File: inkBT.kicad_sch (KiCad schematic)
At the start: 34 parts, among them J1 AudioJack2_Ground, J2 Conn_01x10, J3 Conn_01x06, U1 LM2596S-5, U2 ESP32-WROOM-32, U3 PCM5102A, U5 LM2596S-3.3, U6 ME6211C33M5, U7 ME6211C33M5

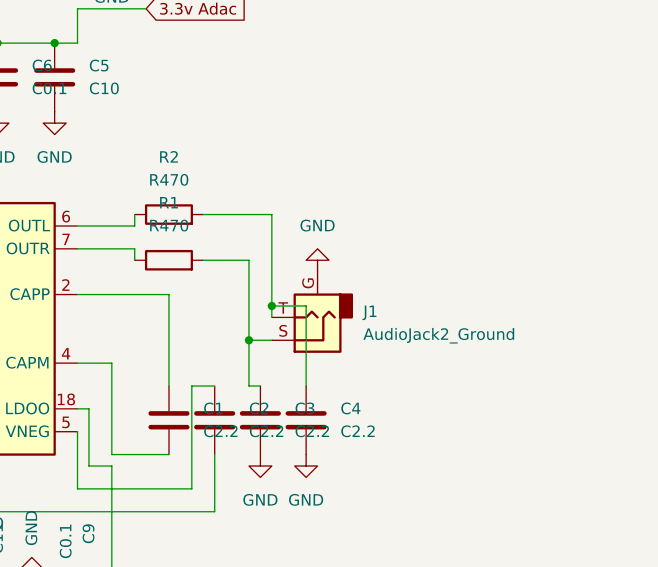
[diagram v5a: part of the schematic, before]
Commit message: a
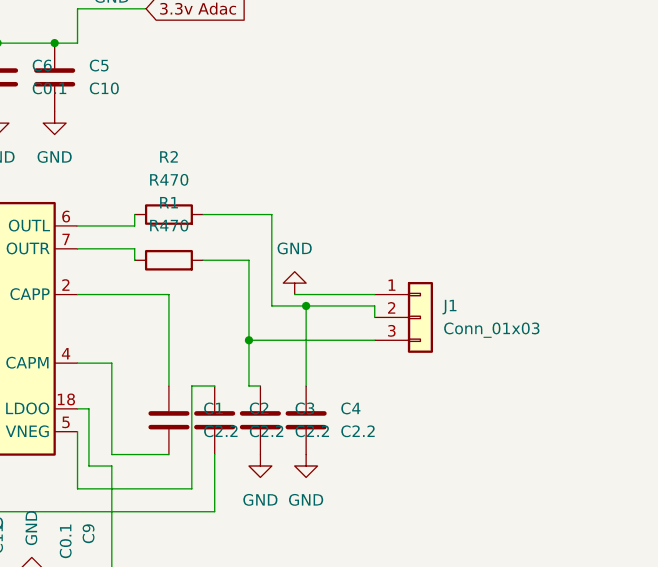
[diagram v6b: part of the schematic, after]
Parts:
- removed J1: AudioJack2_Ground, Connector_PinSocket_1.00mm:PinSocket_1x03_P1.00mm_Vertical, symbol Connector_Audio:AudioJack2_Ground
- added J1: Conn_01x03, Connector_PinHeader_2.00mm:PinHeader_1x03_P2.00mm_Vertical, symbol Connector_Generic:Conn_01x03
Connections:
- net GND: now also J1.1 (Pin_1)
- net at C3.1, R1.2: now also J1.3 (Pin_3)
- net at C4.1, R2.2: now also J1.2 (Pin_2)
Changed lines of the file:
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@@
 	)
 	(junction
+		(at 157.48 104.14)
+		(diameter 0)
+		(color 0 0 0 0)
+	)
+	(junction
 		(at 123.19 74.93)
 		(diameter 0)
@@
 	)
 	(junction
-		(at 153.67 104.14)
-		(diameter 0)
-		(color 0 0 0 0)
-	)
-	(junction
 		(at 129.54 74.93)
 		(diameter 0)
@@
 	(wire
 		(pts
+			(xy 165.1 104.14) (xy 157.48 104.14)
+		)
+		(stroke
+			(width 0)
+			(type default)
+		)
+	)
+	(wire
+		(pts
 			(xy 121.92 81.28) (xy 119.38 81.28)
 		)
@@
 	(wire
 		(pts
+			(xy 156.21 102.87) (xy 165.1 102.87)
+		)
+		(stroke
+			(width 0)
+			(type default)
+		)
+	)
+	(wire
+		(pts
 			(xy 127 40.64) (xy 127 22.86)
 		)
@@
 	(wire
 		(pts
-			(xy 153.67 104.14) (xy 153.67 105.41)
+			(xy 165.1 104.14) (xy 165.1 105.41)
 		)
 		(stroke
@@
 	(wire
 		(pts
+			(xy 157.48 104.14) (xy 153.67 104.14)
+		)
+		(stroke
+			(width 0)
+			(type default)
+		)
+	)
+	(wire
+		(pts
 			(xy 116.84 123.19) (xy 116.84 127)
 		)
@@
 	(wire
 		(pts
-			(xy 151.13 107.95) (xy 153.67 107.95)
+			(xy 151.13 107.95) (xy 165.1 107.95)
 		)
 		(stroke
@@
 	(wire
 		(pts
-			(xy 157.48 104.14) (xy 153.67 104.14)
-		)
-		(stroke
-			(width 0)
-			(type default)
-		)
-	)
-	(wire
-		(pts
 			(xy 97.79 100.33) (xy 106.68 100.33)
 		)
@@
 		(lib_name "GND_1")
 		(lib_id "power:GND")
-		(at 158.75 100.33 180)
+		(at 156.21 102.87 180)
 		(unit 1)
 		(body_style 1)
@@
 		(fields_autoplaced yes)
 		(property "Reference" "#PWR05"
-			(at 158.75 93.98 0)
+			(at 156.21 96.52 0)
 			(hide yes)
 			(show_name no)
@@
 		)
 		(property "Value" "GND"
-			(at 158.75 95.25 0)
+			(at 156.21 97.79 0)
 			(show_name no)
 			(do_not_autoplace no)
@@
 		)
 		(property "Footprint" ""
-			(at 158.75 100.33 0)
+			(at 156.21 102.87 0)
 			(hide yes)
 			(show_name no)
@@
 		)
 		(property "Datasheet" ""
-			(at 158.75 100.33 0)
+			(at 156.21 102.87 0)
 			(hide yes)
 			(show_name no)
@@
 		)
 		(property "Description" "Power symbol creates a global label with name \"GND\" , ground"
-			(at 158.75 100.33 0)
+			(at 156.21 102.87 0)
 			(hide yes)
 			(show_name no)
@@
 	)
 	(symbol
+		(lib_id "Connector_Generic:Conn_01x03")
+		(at 170.18 105.41 0)
+		(unit 1)
+		(body_style 1)
+		(exclude_from_sim no)
+		(in_bom yes)
+		(on_board yes)
+		(in_pos_files yes)
+		(dnp no)
+		(fields_autoplaced yes)
+		(property "Reference" "J1"
+			(at 172.72 104.1399 0)
+			(show_name no)
+			(do_not_autoplace no)
+			(effects
+				(font
+					(size 1.27 1.27)
+				)
+				(justify left)
+			)
+		)
+		(property "Value" "Conn_01x03"
+			(at 172.72 106.6799 0)
+			(show_name no)
+			(do_not_autoplace no)
+			(effects
+				(font
+					(size 1.27 1.27)
+				)
+				(justify left)
+			)
+		)
+		(property "Footprint" "Connector_PinHeader_2.00mm:PinHeader_1x03_P2.00mm_Vertical"
+			(at 170.18 105.41 0)
+			(hide yes)
+			(show_name no)
+			(do_not_autoplace no)
+			(effects
+				(font
+					(size 1.27 1.27)
+				)
+			)
+		)
+		(property "Datasheet" ""
+			(at 170.18 105.41 0)
+			(hide yes)
+			(show_name no)
+			(do_not_autoplace no)
+			(effects
+				(font
+					(size 1.27 1.27)
+				)
+			)
+		)
+		(property "Description" "Generic connector, single row, 01x03, script generated (kicad-library-utils/schlib/autogen/connector/)"
+			(at 170.18 105.41 0)
+			(hide yes)
+			(show_name no)
+			(do_not_autoplace no)
+			(effects
+				(font
+					(size 1.27 1.27)
+				)
+			)
+		)
+		(pin "2"
+		)
+		(pin "1"
+		)
+		(pin "3"
+		)
+		(instances
+			(project "inkBT"
+				(path "/d639bd58-f563-44ff-a906-a8a044dd820d"
+					(reference "J1")
+					(unit 1)
+				)
+			)
+		)
+	)
+	(symbol
 		(lib_id "Device:R")
 		(at 142.24 93.98 90)
@@
 					(unit 1)
 				)
-			)
-		)
-	)
-	(symbol
-		(lib_id "Connector_Audio:AudioJack2_Ground")
-		(at 158.75 105.41 180)
-		(unit 1)
-		(body_style 1)
-		(exclude_from_sim no)
-		(in_bom yes)
-		(on_board yes)
-		(in_pos_files yes)
-		(dnp no)
-		(fields_autoplaced yes)
-		(property "Reference" "J1"
-			(at 163.83 104.775 0)
-			(show_name no)
-			(do_not_autoplace no)
-			(effects
-				(font
-					(size 1.27 1.27)
-				)
-				(justify right)
-			)
-		)
-		(property "Value" "AudioJack2_Ground"
-			(at 163.83 107.315 0)
-			(show_name no)
-			(do_not_autoplace no)
-			(effects
-				(font
-					(size 1.27 1.27)
-				)
-				(justify right)
-			)
-		)
-		(property "Footprint" "Connector_PinSocket_1.00mm:PinSocket_1x03_P1.00mm_Vertical"
-			(at 158.75 105.41 0)
-			(hide yes)
-			(show_name no)
-			(do_not_autoplace no)
-			(effects
-				(font
-					(size 1.27 1.27)
-				)
-			)
-		)
-		(property "Datasheet" ""
-			(at 158.75 105.41 0)
-			(hide yes)
-			(show_name no)
-			(do_not_autoplace no)
-			(effects
-				(font
-					(size 1.27 1.27)
-				)
-			)
-		)
-		(property "Description" ""
-			(at 158.75 105.41 0)
-			(show_name no)
-			(do_not_autoplace no)
-			(effects
-				(font
-					(size 1.27 1.27)
-				)
-			)
-		)
-		(pin "S"
-		)
-		(pin "G"
-		)
-		(pin "T"
-		)
-		(instances
-			(project "inkBT"
-				(path "/d639bd58-f563-44ff-a906-a8a044dd820d"
-					(reference "J1")
-					(unit 1)
-				)

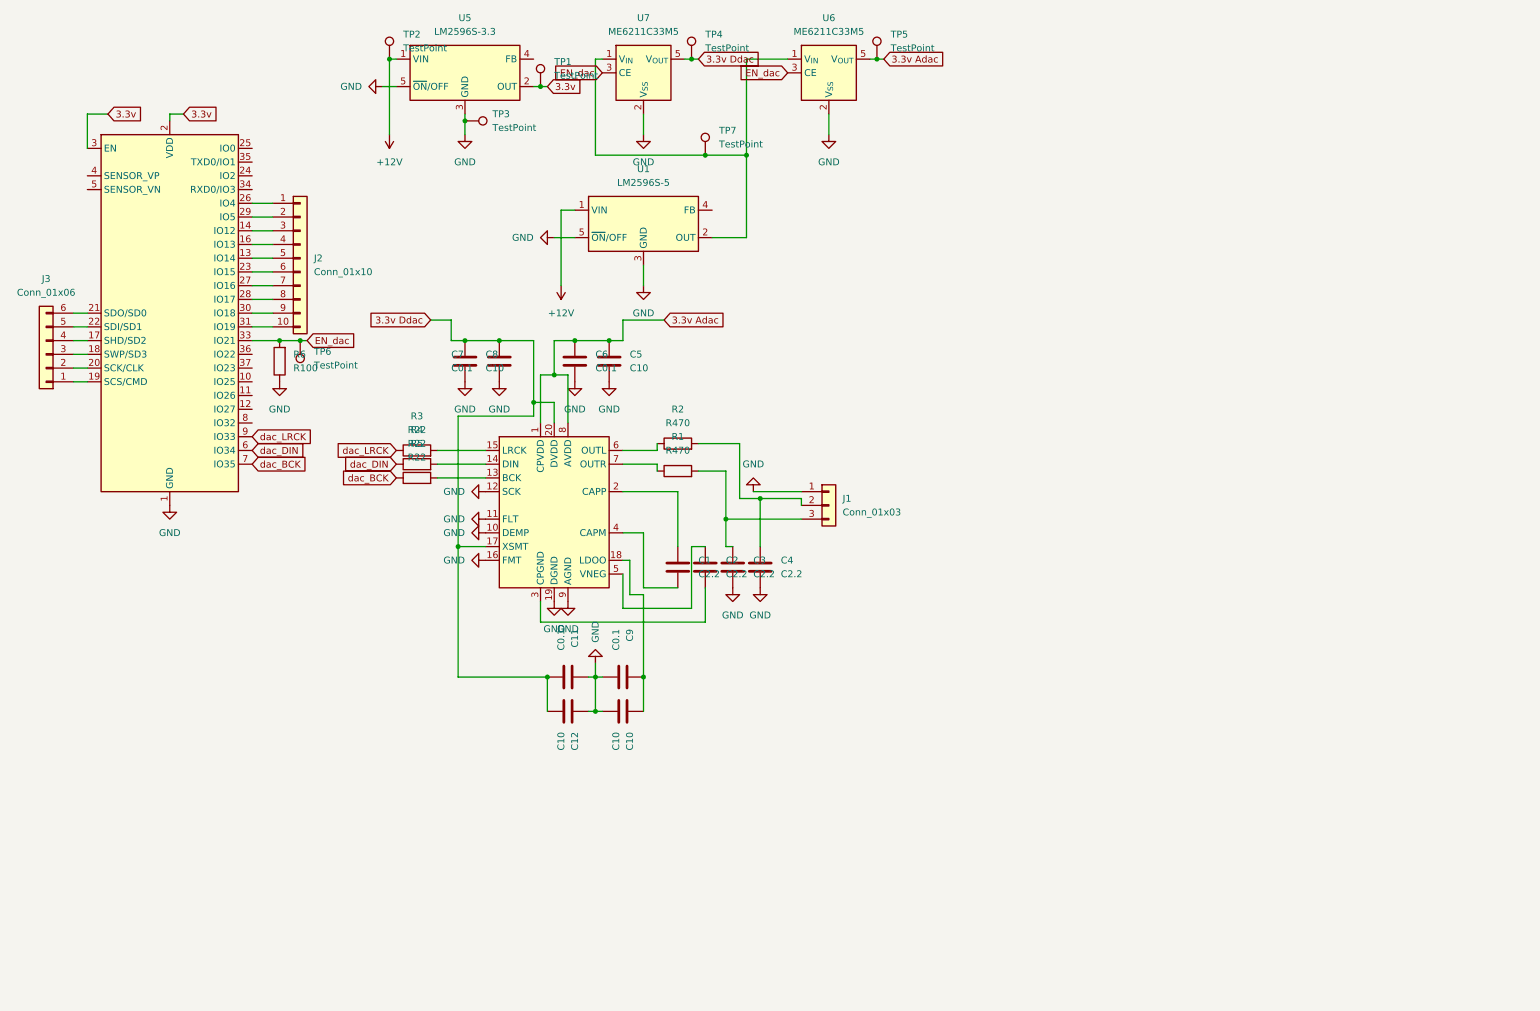
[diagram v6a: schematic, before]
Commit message: a
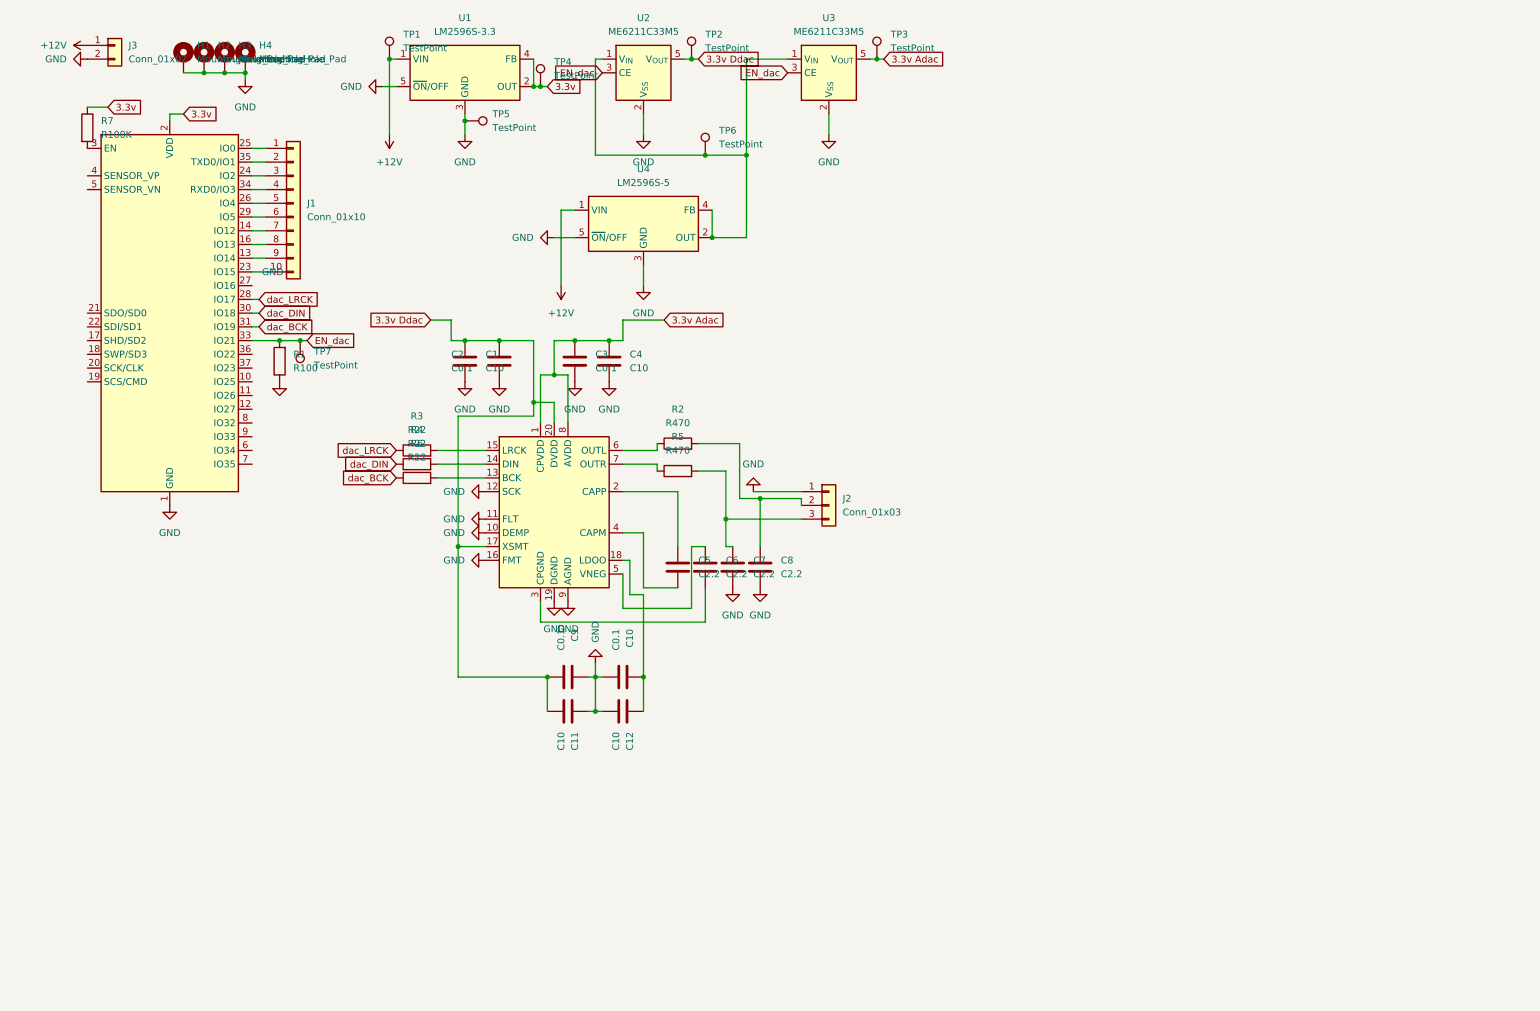
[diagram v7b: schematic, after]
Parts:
- removed J3: Conn_01x06, Connector_PinHeader_2.00mm:PinHeader_1x06_P2.00mm_Vertical, symbol Connector_Generic:Conn_01x06
- added H1, H2, H3, H4: MountingHole_Pad, MountingHole:MountingHole_2.5mm_Pad_Via, symbol Mechanical:MountingHole_Pad
- added J3: Conn_01x02, Connector_PinHeader_2.54mm:PinHeader_1x02_P2.54mm_Vertical, symbol Connector_Generic:Conn_01x02
- added R7: R100K, Resistor_SMD:R_1206_3216Metric_Pad1.30x1.75mm_HandSolder, symbol Device:R
- renumbered C8 to C1, C9 to C10, C12 to C11, C10 to C12, C7 to C2, C6 to C3, C5 to C4, C1 to C5, C2 to C6, C3 to C7, C4 to C8, C11 to C9, J2 to J1, J1 to J2, R6 to R1, R1 to R5, R5 to R6, TP2 to TP1, TP4 to TP2, TP5 to TP3, TP1 to TP4, TP3 to TP5, TP7 to TP6, TP6 to TP7, U5 to U1, U7 to U2, U6 to U3, U1 to U4, U2 to U5, U3 to U6
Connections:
- net +12V: now also J3.1 (Pin_1)
- net 3.3v: now also U1.4 (FB), R7.1; no longer U5.3 (EN)
- net GND: now also H1.1, H2.1, H3.1, H4.1, J3.2 (Pin_2)
- net dac_BCK: now also U5.31 (IO19); no longer U5.7 (IO35)
- net dac_DIN: now also U5.30 (IO18); no longer U5.6 (IO34)
- net dac_LRCK: now also U5.28 (IO17); no longer U5.9 (IO33)
- net at TP6.1, U2.1 (V_{IN}), U3.1 (V_{IN})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: now also U4.4 (FB)
- net at J1.1 (Pin_1): now also U5.25 (IO0); no longer U5.26 (IO4)
- net at J1.10 (Pin_10): now also U5.23 (IO15); no longer U5.31 (IO19)
- net at J1.2 (Pin_2): now also U5.35 (TXD0/IO1); no longer U5.29 (IO5)
- net at J1.3 (Pin_3): now also U5.24 (IO2); no longer U5.14 (IO12)
- net at J1.4 (Pin_4): now also U5.34 (RXD0/IO3); no longer U5.16 (IO13)
- net at J1.5 (Pin_5): now also U5.26 (IO4); no longer U5.13 (IO14)
- net at J1.6 (Pin_6): now also U5.29 (IO5); no longer U5.23 (IO15)
- net at J1.7 (Pin_7): now also U5.14 (IO12); no longer U5.27 (IO16)
- net at J1.8 (Pin_8): now also U5.16 (IO13); no longer U5.28 (IO17)
- net at J1.9 (Pin_9): now also U5.13 (IO14); no longer U5.30 (IO18)
- new net: R7.2, U5.3 (EN)
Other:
- moved on the sheet: J1

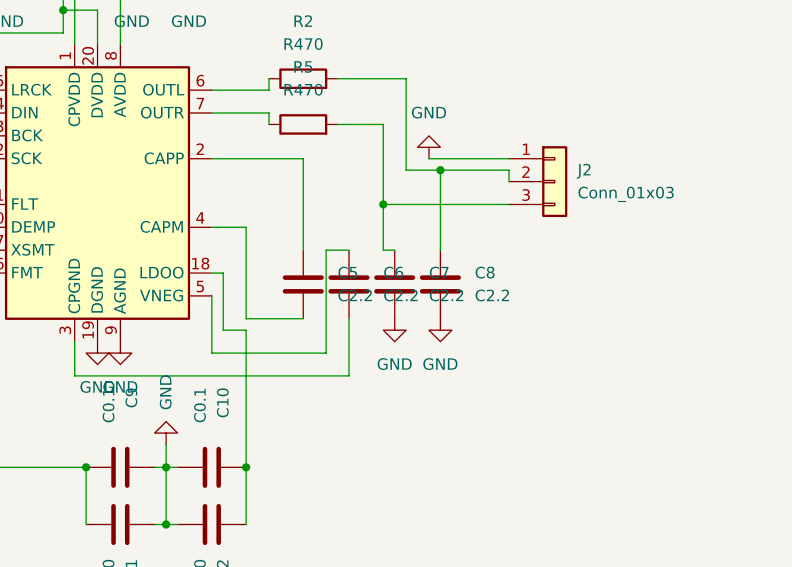
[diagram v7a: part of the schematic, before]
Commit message: a
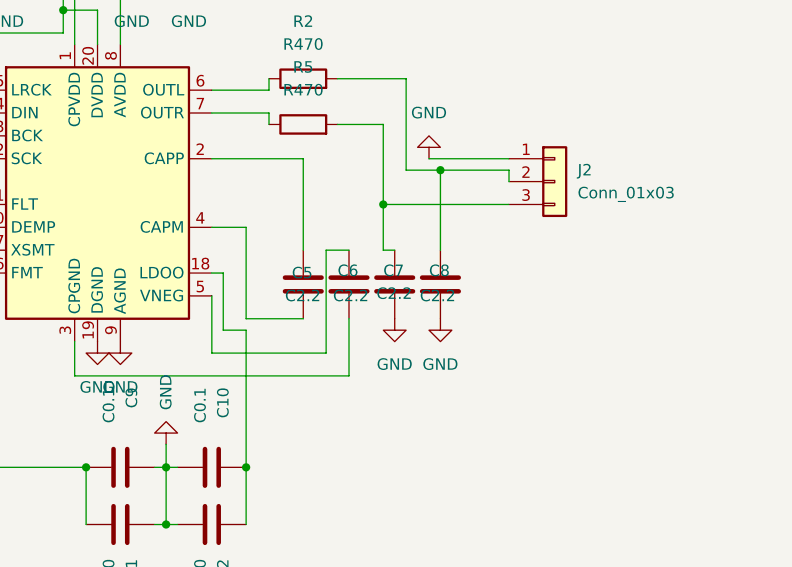
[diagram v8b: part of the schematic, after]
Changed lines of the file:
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@@
 		(in_pos_files yes)
 		(dnp no)
-		(fields_autoplaced yes)
 		(property "Reference" "C7"
-			(at 156.21 115.5699 0)
+			(at 151.13 115.316 0)
 			(show_name no)
 			(do_not_autoplace no)
@@
 		)
 		(property "Value" "C2.2"
-			(at 156.21 118.1099 0)
+			(at 150.368 117.856 0)
 			(show_name no)
 			(do_not_autoplace no)
@@
 		(in_pos_files yes)
 		(dnp no)
-		(fields_autoplaced yes)
 		(property "Reference" "C5"
-			(at 146.05 115.5699 0)
+			(at 140.97 115.57 0)
 			(show_name no)
 			(do_not_autoplace no)
@@
 		)
 		(property "Value" "C2.2"
-			(at 146.05 118.1099 0)
+			(at 140.208 118.11 0)
 			(show_name no)
 			(do_not_autoplace no)
@@
 		(in_pos_files yes)
 		(dnp no)
-		(fields_autoplaced yes)
 		(property "Reference" "C6"
-			(at 151.13 115.5699 0)
+			(at 146.05 115.316 0)
 			(show_name no)
 			(do_not_autoplace no)
@@
 		)
 		(property "Value" "C2.2"
-			(at 151.13 118.1099 0)
+			(at 145.542 118.11 0)
 			(show_name no)
 			(do_not_autoplace no)
@@
 		(in_pos_files yes)
 		(dnp no)
-		(fields_autoplaced yes)
 		(property "Reference" "C8"
-			(at 161.29 115.5699 0)
+			(at 156.21 115.316 0)
 			(show_name no)
 			(do_not_autoplace no)
@@
 		)
 		(property "Value" "C2.2"
-			(at 161.29 118.1099 0)
-			(show_name no)
-			(do_not_autoplace no)
+			(at 155.194 118.11 0)
+			(show_name no)
+			(do_not_autoplace no)
